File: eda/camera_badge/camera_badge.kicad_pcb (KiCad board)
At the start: 2 copper layers, 111.7 x 76.2 mm, 2 parts, among them U1 ESP32-WROOM-32-DEVKIT

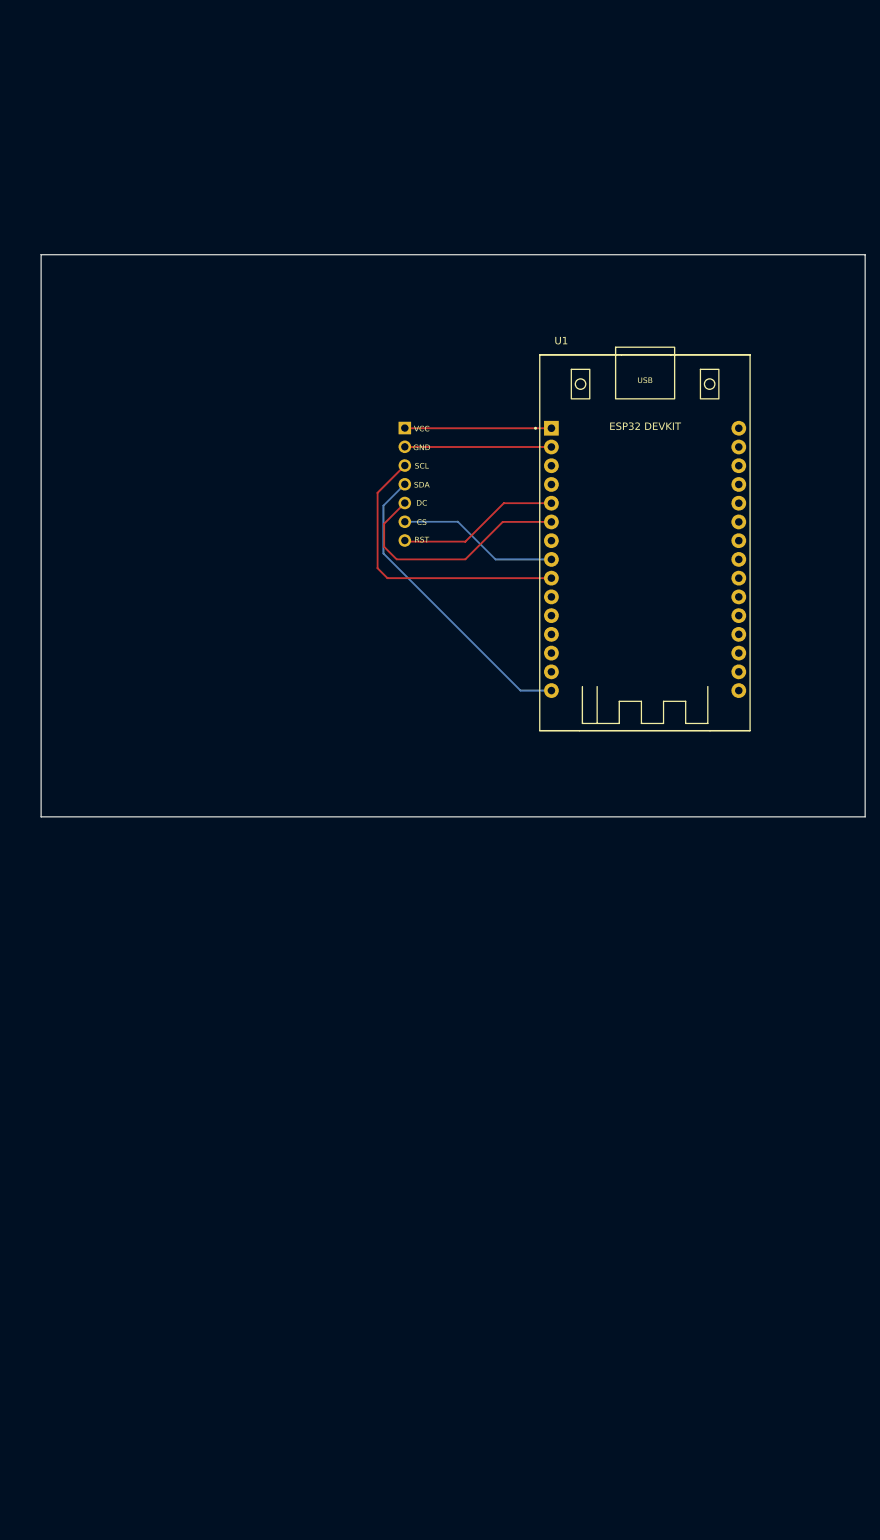
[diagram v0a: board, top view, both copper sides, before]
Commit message: badge eda updates
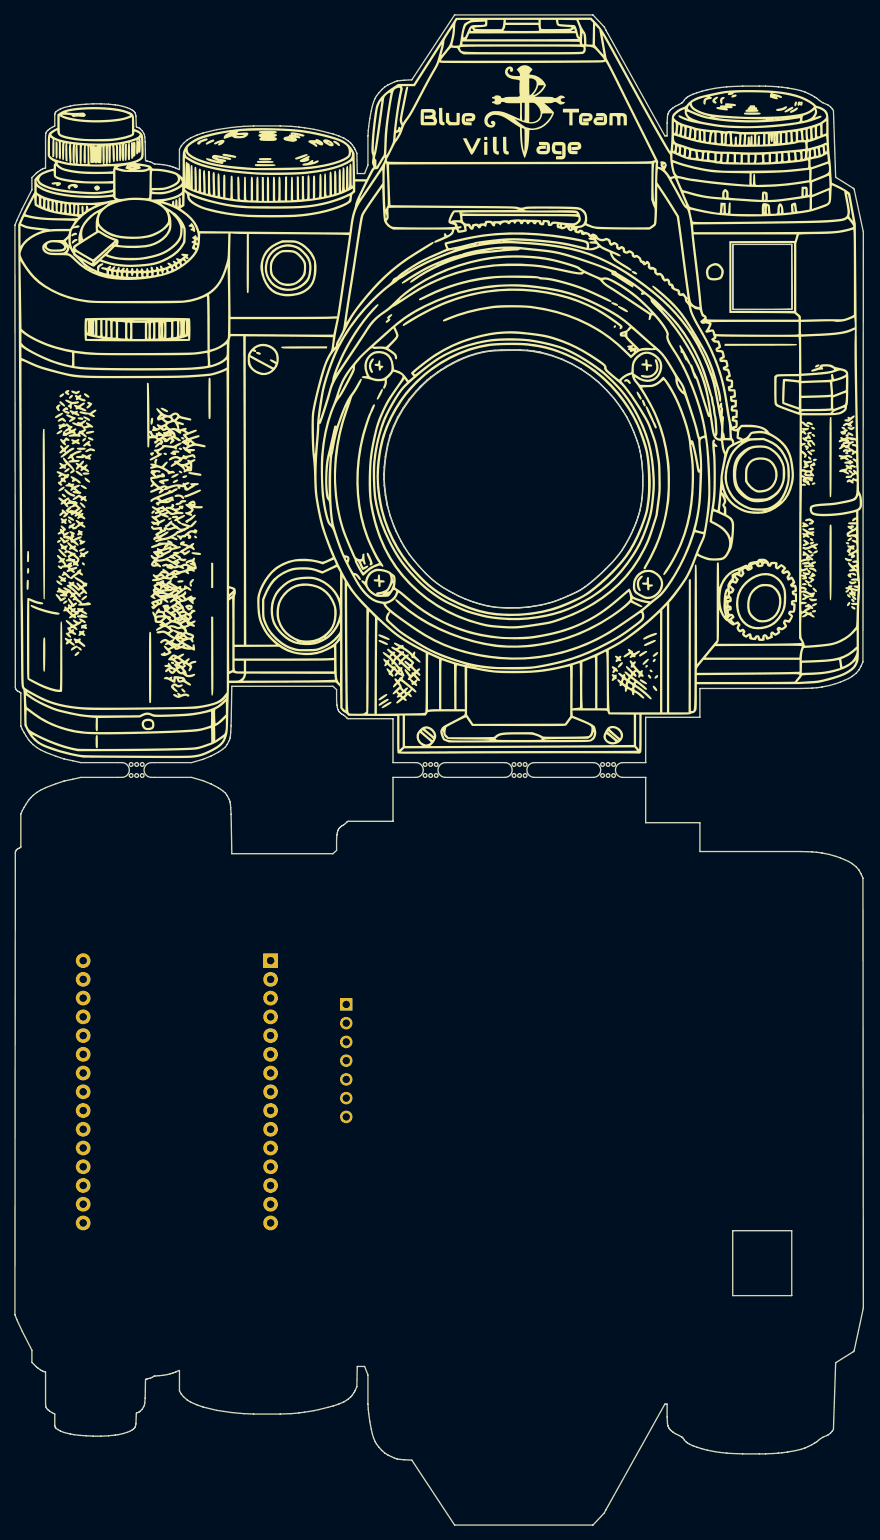
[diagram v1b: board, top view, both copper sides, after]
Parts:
- added G***: Silk01, 0_badge:camera_badge_silk01, F.Cu at (97.3, 123.4)
- added G***: Edge, 0_badge:camera_badge_edgecuts, F.Cu at (97.2, 123.3)
- DS1: footprint 0_local:GC9A01_TFT -> 0_local:GC9A01_TFT_Back_Mount
- U1: footprint 0_local:ESP32_DEVKIT_V1 -> 0_local:ESP32_DEVKIT_V1_Back_Mount
- moved U1 96.1 mm to (61.7, 165.2)
- moved DS1 78.5 mm to (84.7, 155.6)
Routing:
- net D23: track 41.0 -> 0.00 mm
- net D18: track 39.6 -> 0.00 mm
- net D16: track 32.6 -> 0.00 mm
- net D4: track 22.1 -> 0.00 mm
- net D5: track 22.0 -> 0.00 mm
- net +3.3V: track 19.9 -> 0.00 mm
- net GND: track 19.9 -> 0.00 mm
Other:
- board size 111.7 x 76.2 mm -> 115 x 204.7 mm

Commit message: eda update
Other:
- board text added: "-- Inside --"
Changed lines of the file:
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@@
     (property "ki_keywords" "GC9A01 TFT Display")
     (attr through_hole)
-    (fp_text reference "DS1" (at -1.5 -2.7) (layer "B.SilkS")
+    (fp_text reference "DS1" (at -1.96 -5.33 180 unlocked) (layer "B.SilkS")
         (effects (font (size 1 1) (thickness 0.15)) (justify mirror))
     )
     (fp_text value "GC9A01 TFT Display" (at 23.25 15.55) (layer "B.Fab")
-        (effects (font (size 1 1) (thickness 0.15)) (justify mirror))
+        (effects (font (size 1 1) (thickness 0.15)))
     )
-    (fp_text user "SCL" (at -2.3 5.15) (layer "B.SilkS")
+    (fp_text user "SCL" (at -2.3 5.15 180 unlocked) (layer "B.SilkS")
         (effects (font (size 0.75 0.75) (thickness 0.15)) (justify mirror))
     )
-    (fp_text user "GND" (at -2.3 2.65) (layer "B.SilkS")
+    (fp_text user "GND" (at -2.3 2.65 180 unlocked) (layer "B.SilkS")
         (effects (font (size 0.75 0.75) (thickness 0.15)) (justify mirror))
     )
-    (fp_text user "CS" (at -2.3 12.78) (layer "B.SilkS")
+    (fp_text user "CS" (at -2.3 12.78 180 unlocked) (layer "B.SilkS")
         (effects (font (size 0.75 0.75) (thickness 0.15)) (justify mirror))
     )
-    (fp_text user "DC" (at -2.3 10.18) (layer "B.SilkS")
+    (fp_text user "DC" (at -2.3 10.18 180 unlocked) (layer "B.SilkS")
         (effects (font (size 0.75 0.75) (thickness 0.15)) (justify mirror))
     )
-    (fp_text user "SDA" (at -2.3 7.72) (layer "B.SilkS")
+    (fp_text user "SDA" (at -2.3 7.72 180 unlocked) (layer "B.SilkS")
         (effects (font (size 0.75 0.75) (thickness 0.15)) (justify mirror))
     )
-    (fp_text user "RST" (at -2.3 15.15) (layer "B.SilkS")
+    (fp_text user "RST" (at -2.3 15.15 180 unlocked) (layer "B.SilkS")
         (effects (font (size 0.75 0.75) (thickness 0.15)) (justify mirror))
     )
-    (fp_text user "VCC" (at -2.3 0.11) (layer "B.SilkS")
+    (fp_text user "VCC" (at -2.3 0.11 180 unlocked) (layer "B.SilkS")
         (effects (font (size 0.75 0.75) (thickness 0.15)) (justify mirror))
     )
@@
     (property "ki_keywords" "RF Radio BT ESP ESP32 Espressif onboard PCB antenna")
     (attr through_hole)
-    (fp_text reference "U1" (at -11.355 -27.36) (layer "B.SilkS")
+    (fp_text reference "U1" (at -11.355 -27.36 180 unlocked) (layer "B.SilkS")
         (effects (font (size 1 1) (thickness 0.15)) (justify mirror))
     )
     (fp_text value "ESP32-WROOM-32-DEVKIT" (at -0.56 27.36) (layer "B.Fab")
-        (effects (font (size 1 1) (thickness 0.15)) (justify mirror))
+        (effects (font (size 1 1) (thickness 0.15)))
     )
-    (fp_text user "ESP32 DEVKIT" (at 0 -15.75 unlocked) (layer "B.SilkS")
+    (fp_text user "ESP32 DEVKIT" (at 0 -15.75 180 unlocked) (layer "B.SilkS")
         (effects (font (size 1 1) (thickness 0.15)) (justify mirror))
     )
-    (fp_text user "USB" (at 0 -22 unlocked) (layer "B.SilkS")
+    (fp_text user "USB" (at 0 -22 180 unlocked) (layer "B.SilkS")
         (effects (font (size 0.75 0.75) (thickness 0.1)) (justify mirror))
     )
@@
     (pad "" np_thru_hole circle (at 23.65 1.25) (size 0.5 0.5) (drill 0.5) (layers "*.Cu" "*.Mask"))
   )
+  (gr_text "-- Inside --" (at 113.8 122) (layer "B.SilkS")
+    (effects (font (size 1 1) (thickness 0.15)) (justify left bottom mirror))
+  )
+  (gr_text "-- Inside --" (at 102.7 125.9 180) (layer "B.SilkS")
+    (effects (font (size 1 1) (thickness 0.15)) (justify left bottom mirror))
+  )
 )
